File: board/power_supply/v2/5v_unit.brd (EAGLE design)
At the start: 25.1 x 51.4 mm, 12 parts

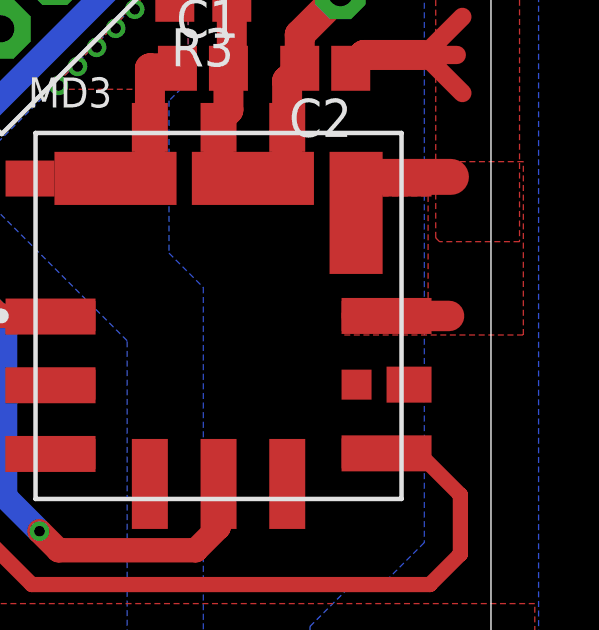
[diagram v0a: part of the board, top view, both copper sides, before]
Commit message: Revert "Merge remote-tracking branch 'origin/Develop' into feature_#37"
This reverts commit cb103155361e8766478c6830db153463370c0739, reversing
changes made to 84e093fe944e1f8653a6822ff34e6f8740617cb5.
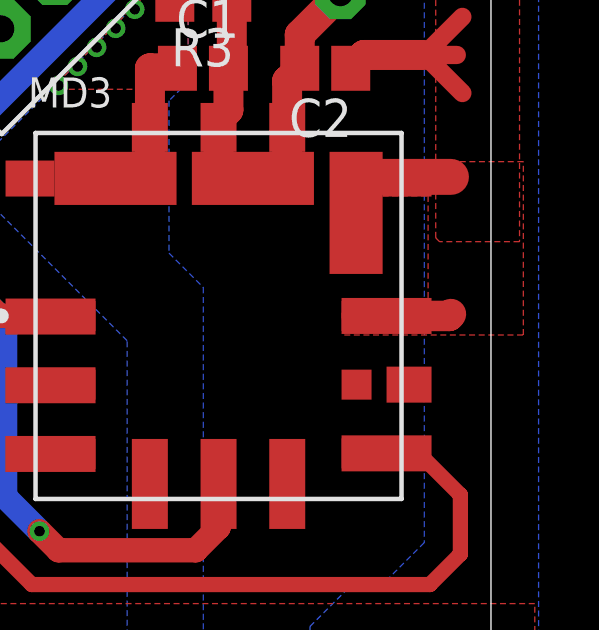
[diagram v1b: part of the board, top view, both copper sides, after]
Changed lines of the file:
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@@
 <?xml version="1.0" encoding="utf-8"?>
 <!DOCTYPE eagle SYSTEM "eagle.dtd">
-<eagle version="9.6.1">
+<eagle version="9.6.2">
 <drawing>
 <settings>
@@
 </layers>
 <board>
-<fusionsync huburn="a.cGVyc29uYWw6dWUyYjhiNWJj" projecturn="a.cGVyc29uYWw6dWUyYjhiNWJjIzIwMjIwNDE2NTE3MzEzNjU2" f3durn="urn:adsk.wipprod:dm.lineage:J4KWdsV-RwmCOziydWyP5A" pcbguid="" lastpulledtime="" lastsyncedchangeguid="" latestrevisionid="46676070-bb23-41f3-9839-3d353bdf0556" lastsyncedrevisionid="46676070-bb23-41f3-9839-3d353bdf0556" lastboardhashguid="7af40513-0a80-27c1-dc80-51a4a12e53d5" lastpushedtime="2022-10-04T02:11:47Z" linktopcb3d="%12"/>
+<fusionsync huburn="a.cGVyc29uYWw6dWUyYjhiNWJj" projecturn="a.cGVyc29uYWw6dWUyYjhiNWJjIzIwMjIwNDE2NTE3MzEzNjU2" f3durn="urn:adsk.wipprod:dm.lineage:J4KWdsV-RwmCOziydWyP5A" pcbguid="" lastpulledtime="" lastsyncedchangeguid="" latestrevisionid="46676070-bb23-41f3-9839-3d353bdf0556" lastsyncedrevisionid="46676070-bb23-41f3-9839-3d353bdf0556" lastboardhashguid="7af40513-0a80-27c1-dc80-51a4a12e53d5" lastpushedtime="2022-10-04T02:11:47Z" linktopcb3d="true"/>
 <plain>
 <circle x="23.083259375" y="2.542159375" radius="1.05" width="0.001" layer="20"/>
@@
 <wire x1="22.86" y1="30.48" x2="24.13" y2="29.21" width="0.6096" layer="1"/>
 <wire x1="20.602" y1="21.7805" x2="23.6855" y2="21.7805" width="1.016" layer="1"/>
+<wire x1="23.6855" y1="21.7805" x2="23.749" y2="21.844" width="1.016" layer="1"/>
 </signal>
 <signal name="N$9">

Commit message: marge前のファイル
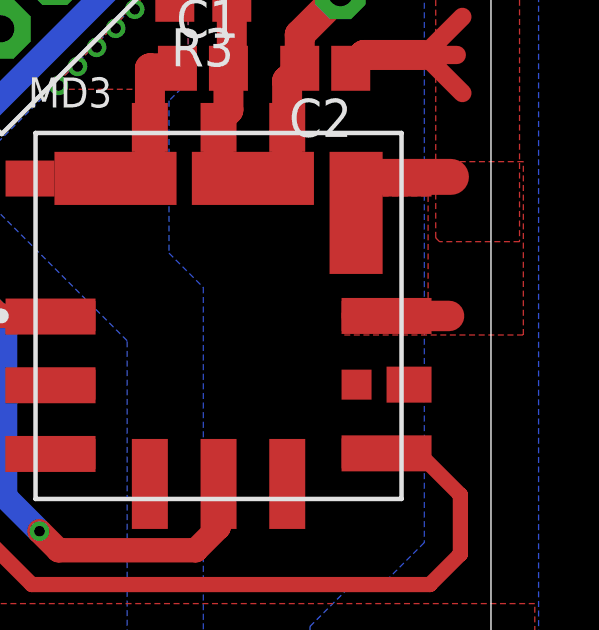
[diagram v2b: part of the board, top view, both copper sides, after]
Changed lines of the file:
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@@
 <wire x1="22.86" y1="30.48" x2="24.13" y2="29.21" width="0.6096" layer="1"/>
 <wire x1="20.602" y1="21.7805" x2="23.6855" y2="21.7805" width="1.016" layer="1"/>
-<wire x1="23.6855" y1="21.7805" x2="23.749" y2="21.844" width="1.016" layer="1"/>
 </signal>
 <signal name="N$9">
